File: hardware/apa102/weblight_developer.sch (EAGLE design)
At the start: 14 parts, among them U1 ATTiny85-20SU

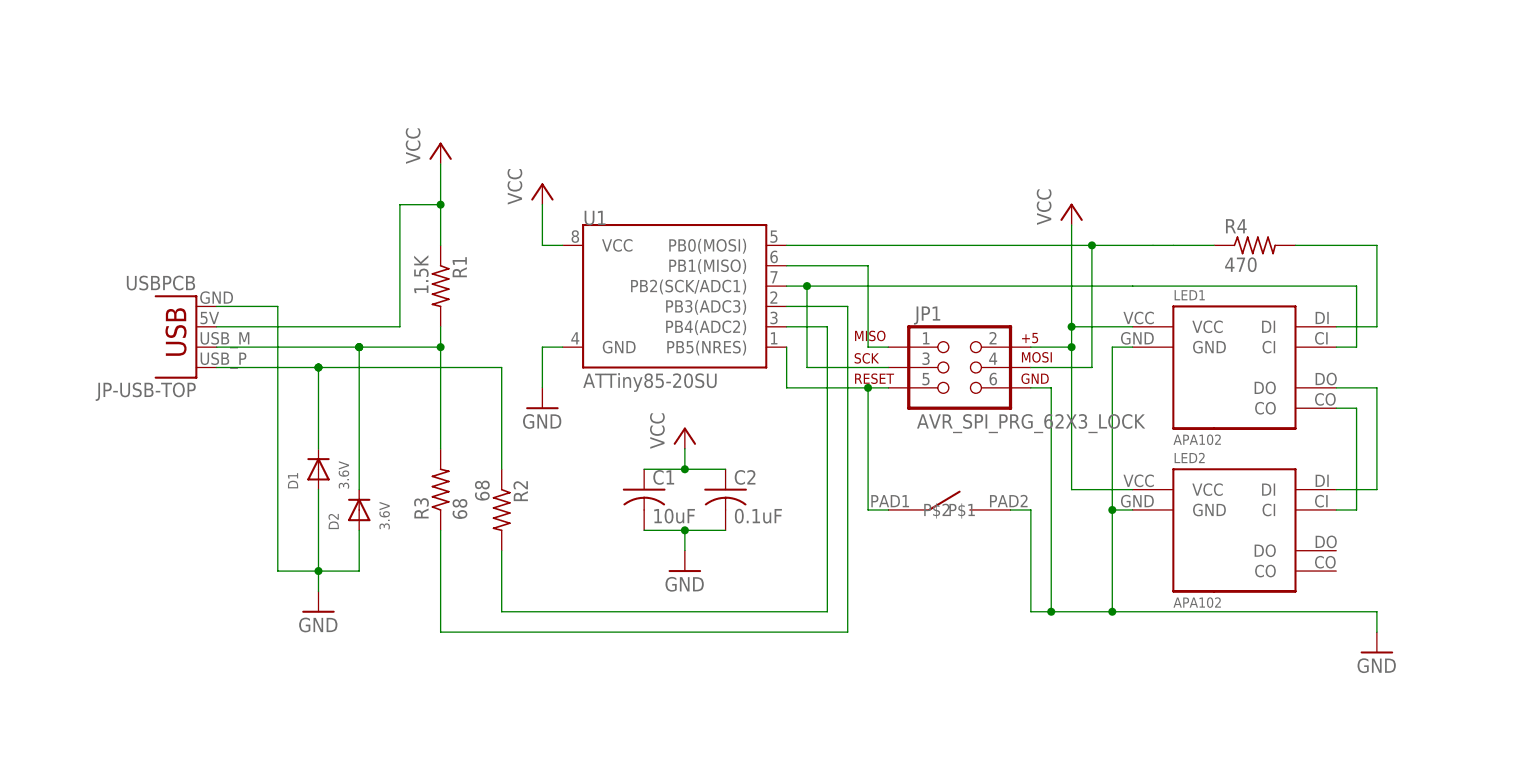
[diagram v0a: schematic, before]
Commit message: a-osh1
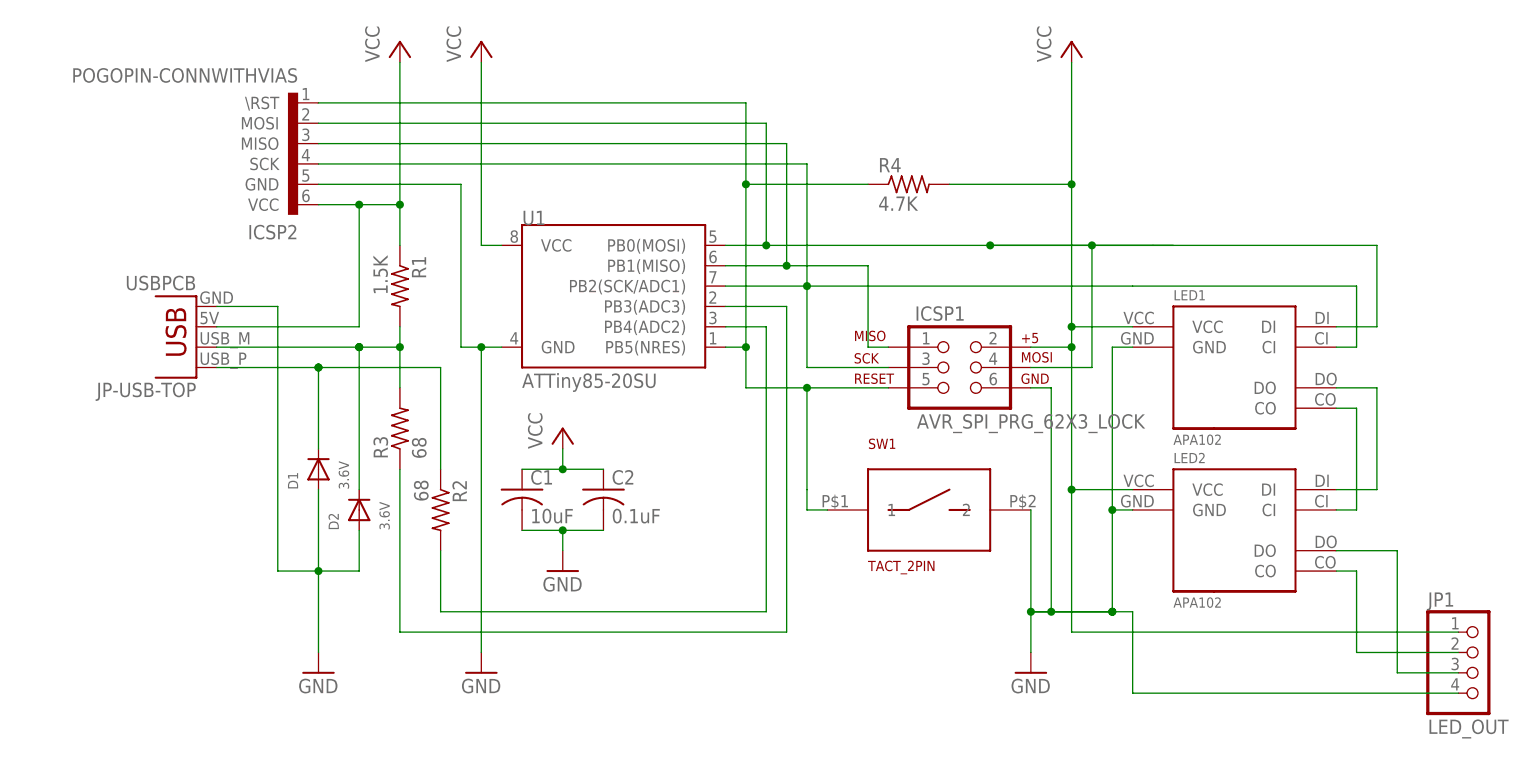
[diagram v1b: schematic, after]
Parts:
- removed SW_RESET: BUTTON_TD-85XU, weblight:BUTTON_TD-85XU
- added ICSP1: AVR_SPI_PRG_62X3_LOCK, SparkFun-Connectors:AVR_SPI_PRG_62X3_LOCK
- added ICSP2: POGOPIN-CONNWITHVIAS, weblight:POGOPIN-CONNWITHVIAS
- added SW1: TACT_2PIN, weblight:TACT_2PIN
- JP1: value AVR_SPI_PRG_62X3_LOCK -> LED_OUT; device SparkFun-Connectors:AVR_SPI_PRG_62X3_LOCK -> microbuilder:HEADER-1X4ROUND
- R4: value 470 -> 4.7K
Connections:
- net DIN_2 renamed DATA_2
- net SCK_2 renamed CLK_2
- removed net DIN_1: LED1.DI, R4.2
- removed net MOSI/DIN_RAW: JP1.4, R4.1, U1.PB0(MOSI)
- removed net RESET: JP1.5, SW_RESET.P$1, U1.PB5(NRES)
- removed net SCK_1: JP1.3, LED1.CI, U1.PB2(SCK/ADC1)
- new net CLK_1/SCK: ICSP1.3, ICSP2.SCK, LED1.CI, U1.PB2(SCK/ADC1)
- new net CLK_3: JP1.2, LED2.CO
- new net DATA_1/MOSI: ICSP1.4, ICSP2.MOSI, LED1.DI, U1.PB0(MOSI)
- new net DATA_3: JP1.3, LED2.DO
- new net N_RESET: ICSP1.5, ICSP2.\RST, R4.1, SW1.1, U1.PB5(NRES)
- net GND: now also ICSP1.6, ICSP2.GND, JP1.4, SW1.2; no longer JP1.6, SW_RESET.P$2
- net MISO: now also ICSP1.1, ICSP2.MISO; no longer JP1.1
- net VCC: now also ICSP1.2, ICSP2.VCC, JP1.1, R4.2; no longer JP1.2
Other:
- moved on the sheet: C1, C2, R1, R2, R3, R4, U1
